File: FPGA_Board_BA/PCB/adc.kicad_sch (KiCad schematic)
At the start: 1 part, among them U1 LTC2320-16

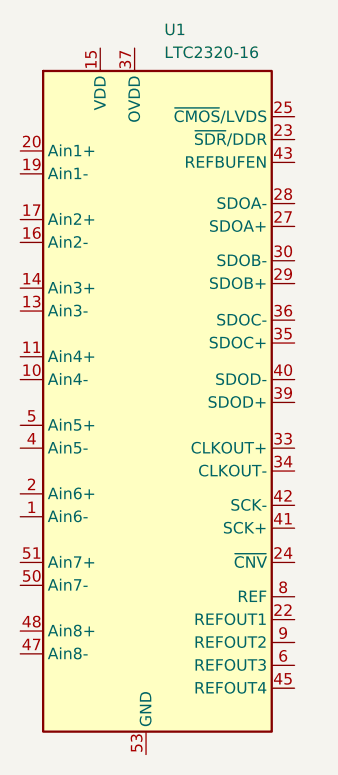
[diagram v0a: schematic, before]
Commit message: some changes + lib
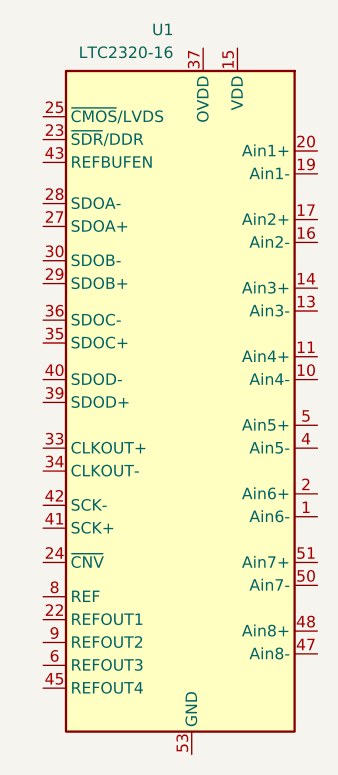
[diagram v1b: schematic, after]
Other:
- moved on the sheet: U1
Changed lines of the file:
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@@
 		(lib_id "MYLIB_U:LTC2320-16")
 		(at 119.38 104.14 0)
+		(mirror y)
 		(unit 1)
 		(exclude_from_sim no)
@@
 		(dnp no)
 		(property "Reference" "U1"
-			(at 118.872 64.008 0)
+			(at 119.888 64.008 0)
 			(effects
 				(font
@@
 		)
 		(property "Value" "LTC2320-16"
-			(at 118.872 66.548 0)
+			(at 119.888 66.548 0)
 			(effects
 				(font
@@
 		)
 		(property "Footprint" "MYLIB_chips:UKG_52_7mm_8mm"
-			(at 116.84 52.07 0)
+			(at 121.92 52.07 0)
 			(effects
 				(font
@@
 		)
 		(property "Datasheet" "https://www.analog.com/media/en/technical-documentation/data-sheets/232016fb.pdf"
-			(at 117.348 54.61 0)
+			(at 121.412 54.61 0)
 			(effects
 				(font
@@
 		)
 		(property "Description" "8 Channel 16 Bit Differential ADC"
-			(at 116.078 49.784 0)
+			(at 122.682 49.784 0)
 			(effects
 				(font

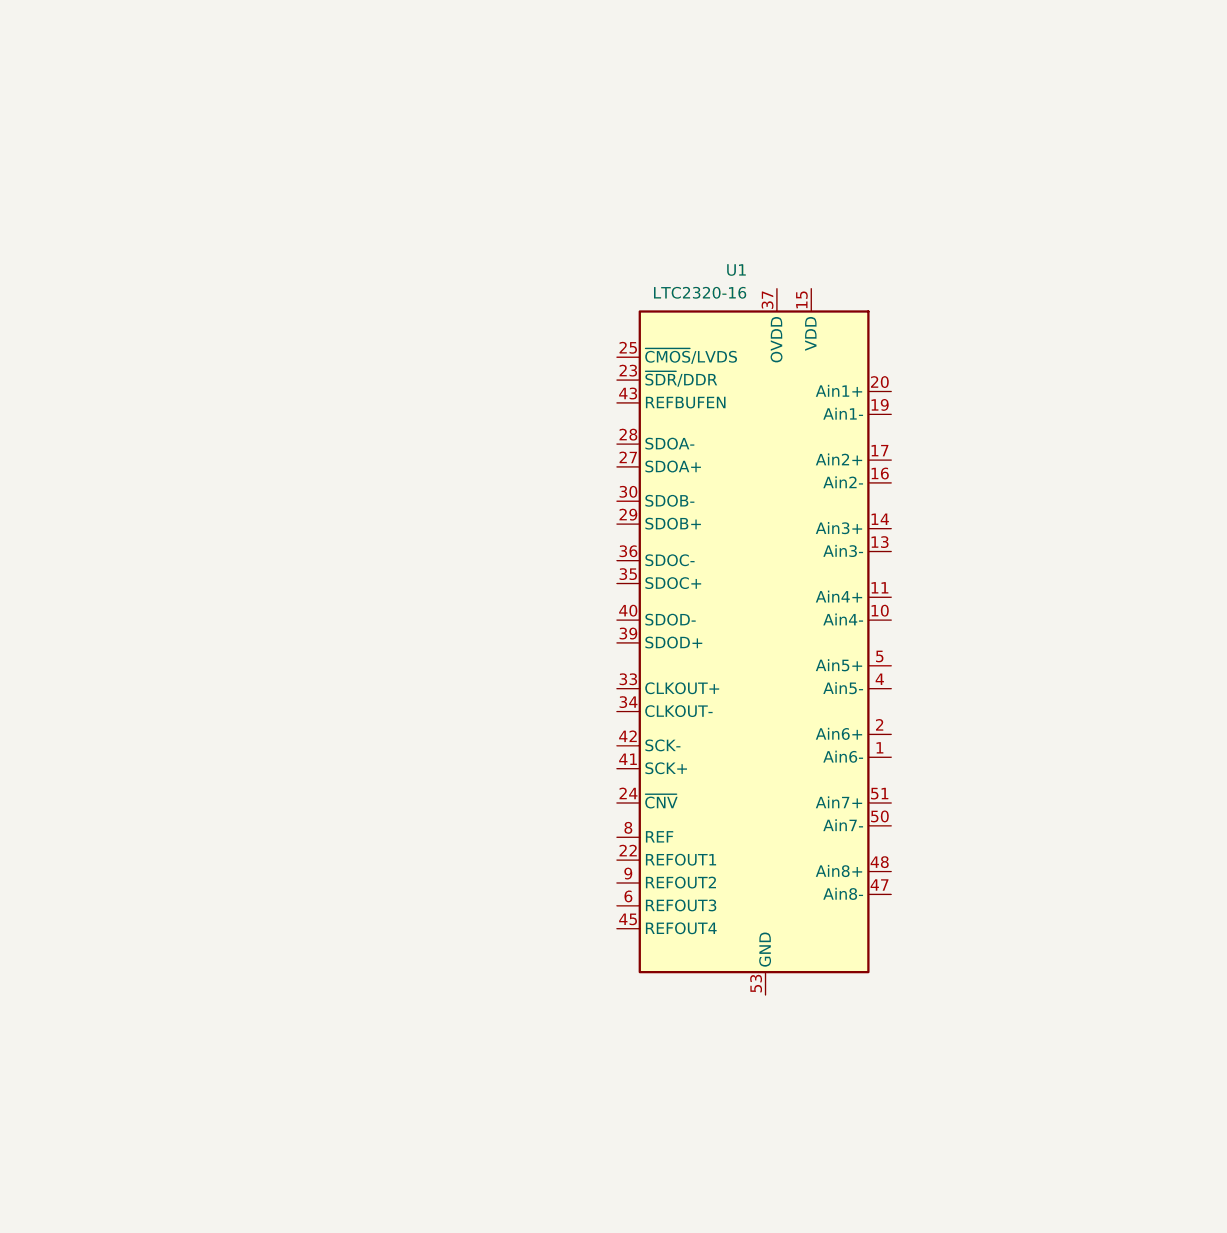
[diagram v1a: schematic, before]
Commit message: schematic almost ready
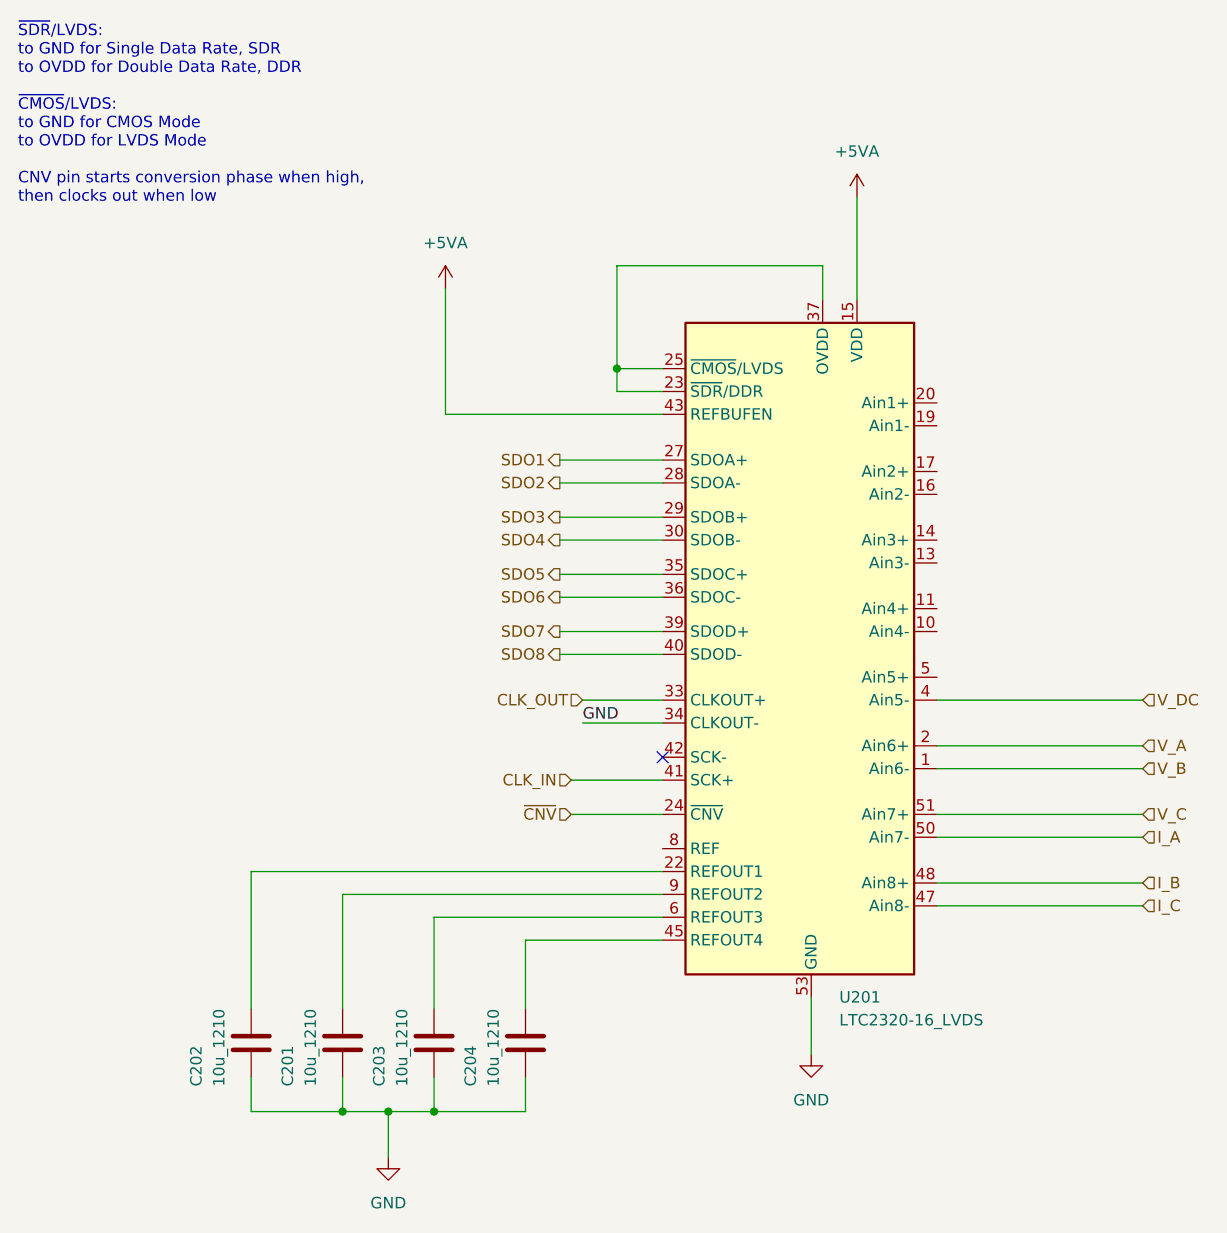
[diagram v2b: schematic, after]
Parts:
- removed U1: LTC2320-16, MYLIB_chips:UKG_52_7mm_8mm, symbol MYLIB_U:LTC2320-16
- added C201, C202, C203, C204: 10u_1210, WLIB_Capacitor:C_1210, symbol WLIB_C:10u_1210
- added U201: LTC2320-16_LVDS, MYLIB_chips:UKG_52_7mm_8mm, symbol MYLIB_U:LTC2320-16_LVDS
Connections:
- net GND: now also C201.2, C202.2, C203.2, C204.2, U201.12 (GND), U201.18 (GND), U201.26 (GND), U201.3 (GND), U201.32 (GND), U201.34 (CLKOUT-), U201.38 (GND), U201.46 (GND), U201.49 (GND), U201.53 (GND), U201.7 (GND)
- net OVDD: now also U201.23 (~{SDR}/DDR), U201.25 (~{CMOS}/LVDS), U201.31 (OVDD), U201.37 (OVDD)
- new net: C203.1, U201.6 (REFOUT3)
- new net: C204.1, U201.45 (REFOUT4)
- new net: C201.1, U201.9 (REFOUT2)
- new net: C202.1, U201.22 (REFOUT1)
- new net +5VA: U201.15 (VDD), U201.21 (VDD), U201.43 (REFBUFEN), U201.44 (VDD), U201.52 (VDD)
- new net CLK_IN: U201.41 (SCK+)
- new net CLK_OUT: U201.33 (CLKOUT+)
- new net I_A: U201.50 (Ain7-)
- new net I_B: U201.48 (Ain8+)
- new net I_C: U201.47 (Ain8-)
- new net SDO1: U201.27 (SDOA+)
- new net SDO2: U201.28 (SDOA-)
- new net SDO3: U201.29 (SDOB+)
- new net SDO4: U201.30 (SDOB-)
- new net SDO5: U201.35 (SDOC+)
- new net SDO6: U201.36 (SDOC-)
- new net SDO7: U201.39 (SDOD+)
- new net SDO8: U201.40 (SDOD-)
- new net V_A: U201.2 (Ain6+)
- new net V_B: U201.1 (Ain6-)
- new net V_C: U201.51 (Ain7+)
- new net V_DC: U201.4 (Ain5-)
- new net ~{CNV}: U201.24 (~{CNV})
- no-connect marks 0 -> 1
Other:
- note added: "~{SDR}/LVDS: to GND for Single Data Rate, SDR to OVDD for Double Data Rate, DDR ~{CMOS}/LVDS: to GND for CMOS Mode to OVDD for LVDS Mode CNV pin starts conversion phase when high, then clocks out when low"
